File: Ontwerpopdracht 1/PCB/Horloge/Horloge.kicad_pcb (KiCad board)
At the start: 2 copper layers, 40 x 40 mm, 49 parts, among them J1 Conn_01x03, Q1 BSS138, U1 TPS613222ADBVT, U2 ATTINY414-SSF, Y1 FX135A-327

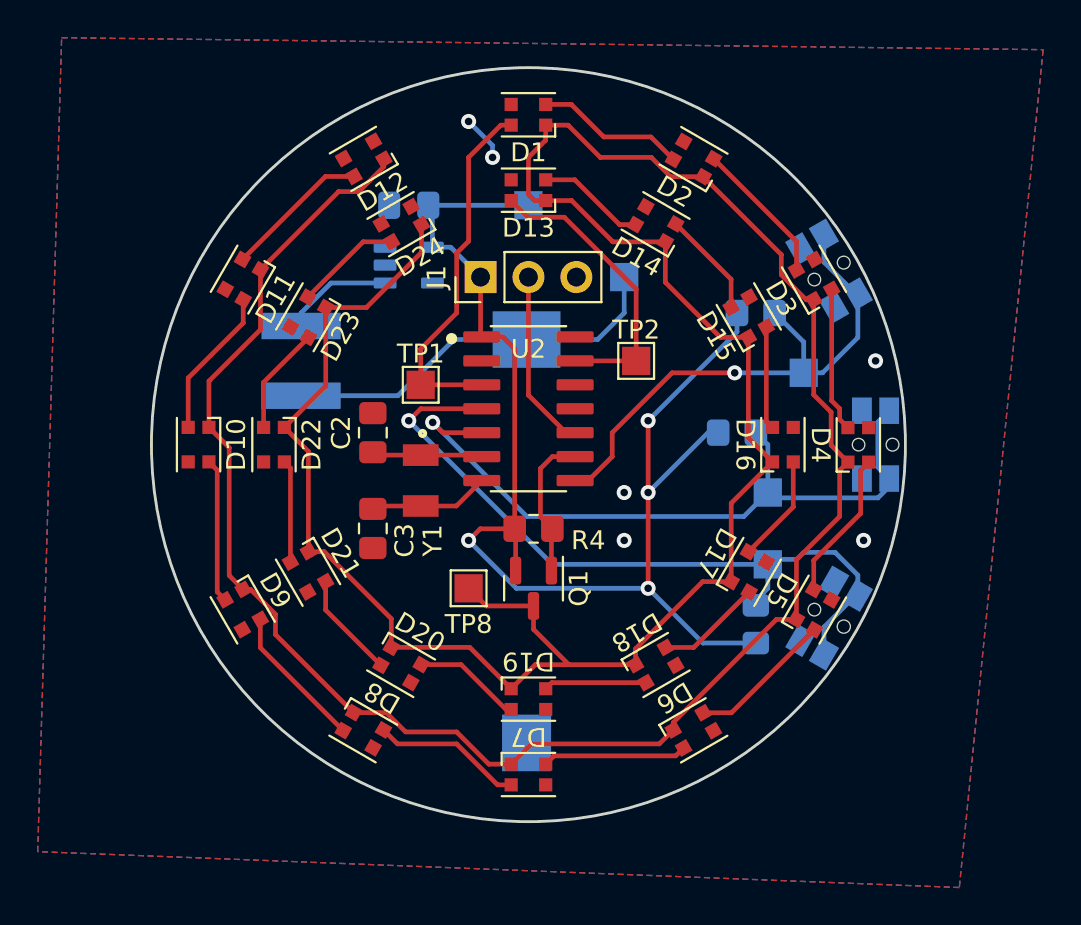
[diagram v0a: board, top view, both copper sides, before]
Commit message: pcb macropad klaar
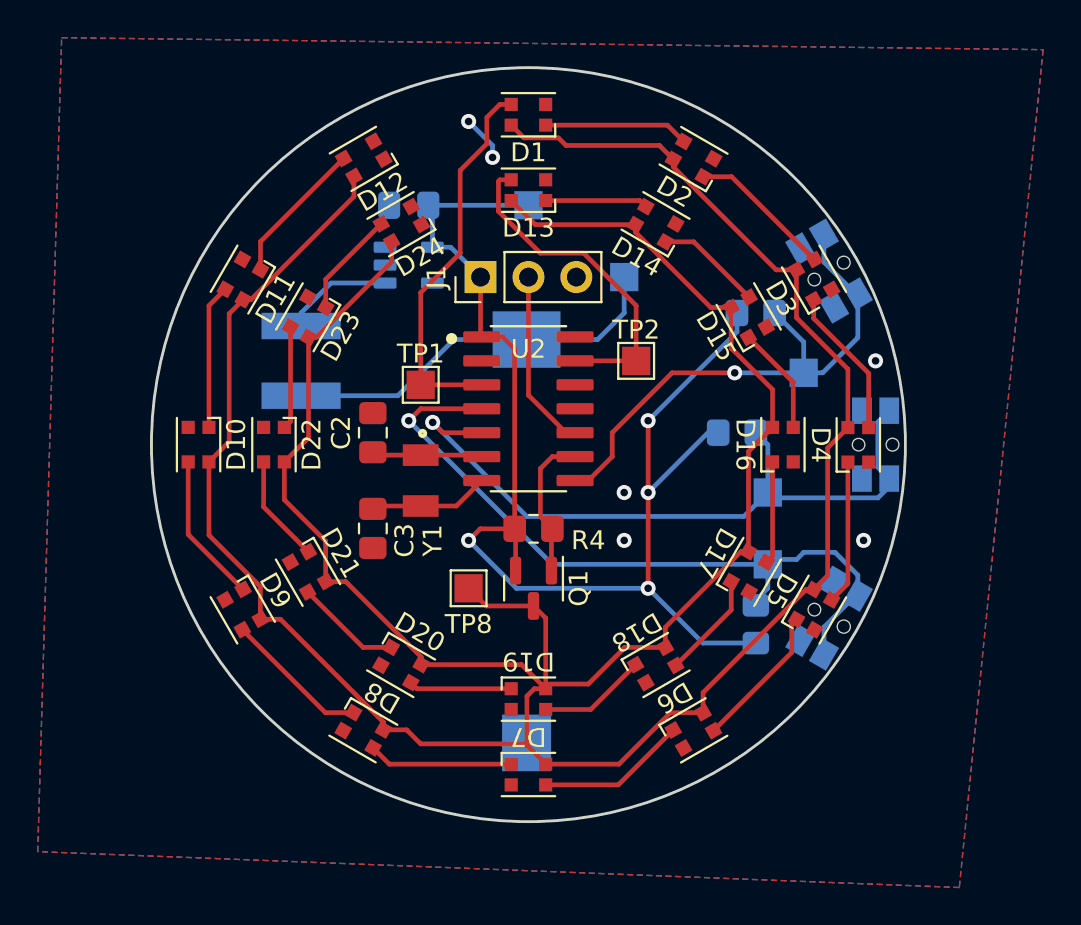
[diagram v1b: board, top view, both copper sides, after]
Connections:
- D1 pad 1: VDD -> Net-(D1-DOUT)
- D1 pad 2: Net-(D1-Pad2) -> GND
- D1 pad 3: GND -> LEDS UREN
- D1 pad 4: LEDS UREN -> VDD
- D10 pad 1: VDD -> Net-(D10-DOUT)
- D10 pad 2: Net-(D10-Pad2) -> GND
- D10 pad 3: GND -> Net-(D10-DIN)
- D10 pad 4: Net-(D10-Pad4) -> VDD
- D11 pad 1: VDD -> Net-(D11-DOUT)
- D11 pad 2: Net-(D11-Pad2) -> GND
- D11 pad 3: GND -> Net-(D10-DOUT)
- D11 pad 4: Net-(D10-Pad2) -> VDD
- D12 pad 1: VDD -> unconnected-(D12-DOUT-Pad1)
- D12 pad 2: unconnected-(D12-Pad2) -> GND
- D12 pad 3: GND -> Net-(D11-DOUT)
- D12 pad 4: Net-(D11-Pad2) -> VDD
- D13 pad 1: VDD -> Net-(D13-DOUT)
- D13 pad 2: Net-(D13-Pad2) -> GND
- D13 pad 3: GND -> LEDS MINUTEN
- D13 pad 4: LEDS MINUTEN -> VDD
- D14 pad 1: VDD -> Net-(D14-DOUT)
- D14 pad 2: Net-(D14-Pad2) -> GND
- D14 pad 3: GND -> Net-(D13-DOUT)
- D14 pad 4: Net-(D13-Pad2) -> VDD
- D15 pad 1: VDD -> Net-(D15-DOUT)
- D15 pad 2: Net-(D15-Pad2) -> GND
- D15 pad 3: GND -> Net-(D14-DOUT)
- D15 pad 4: Net-(D14-Pad2) -> VDD
- D16 pad 1: VDD -> Net-(D16-DOUT)
- D16 pad 2: Net-(D16-Pad2) -> GND
- D16 pad 3: GND -> Net-(D15-DOUT)
- D16 pad 4: Net-(D15-Pad2) -> VDD
- D17 pad 1: VDD -> Net-(D17-DOUT)
- D17 pad 2: Net-(D17-Pad2) -> GND
- D17 pad 3: GND -> Net-(D16-DOUT)
- D17 pad 4: Net-(D16-Pad2) -> VDD
- D18 pad 1: VDD -> Net-(D18-DOUT)
- D18 pad 2: Net-(D18-Pad2) -> GND
- D18 pad 3: GND -> Net-(D17-DOUT)
- D18 pad 4: Net-(D17-Pad2) -> VDD
- D19 pad 1: VDD -> Net-(D19-DOUT)
- D19 pad 2: Net-(D19-Pad2) -> GND
- D19 pad 3: GND -> Net-(D18-DOUT)
- D19 pad 4: Net-(D18-Pad2) -> VDD
- D2 pad 1: VDD -> Net-(D2-DOUT)
- D2 pad 2: Net-(D2-Pad2) -> GND
- D2 pad 3: GND -> Net-(D1-DOUT)
- D2 pad 4: Net-(D1-Pad2) -> VDD
- D20 pad 1: VDD -> Net-(D20-DOUT)
- D20 pad 2: Net-(D20-Pad2) -> GND
- D20 pad 3: GND -> Net-(D19-DOUT)
- D20 pad 4: Net-(D19-Pad2) -> VDD
- D21 pad 1: VDD -> Net-(D21-DOUT)
- D21 pad 2: Net-(D21-Pad2) -> GND
- D21 pad 3: GND -> Net-(D20-DOUT)
- D21 pad 4: Net-(D20-Pad2) -> VDD
- D22 pad 1: VDD -> Net-(D22-DOUT)
- D22 pad 2: Net-(D22-Pad2) -> GND
- D22 pad 3: GND -> Net-(D21-DOUT)
- D22 pad 4: Net-(D21-Pad2) -> VDD
- D23 pad 1: VDD -> Net-(D23-DOUT)
- D23 pad 2: Net-(D23-Pad2) -> GND
- D23 pad 3: GND -> Net-(D22-DOUT)
- D23 pad 4: Net-(D22-Pad2) -> VDD
- D24 pad 1: VDD -> unconnected-(D24-DOUT-Pad1)
- D24 pad 2: unconnected-(D24-Pad2) -> GND
- D24 pad 3: GND -> Net-(D23-DOUT)
- D24 pad 4: Net-(D23-Pad2) -> VDD
- D3 pad 1: VDD -> Net-(D3-DOUT)
- D3 pad 2: Net-(D3-Pad2) -> GND
- D3 pad 3: GND -> Net-(D2-DOUT)
- D3 pad 4: Net-(D2-Pad2) -> VDD
- D4 pad 1: VDD -> Net-(D4-DOUT)
- D4 pad 2: Net-(D4-Pad2) -> GND
- D4 pad 3: GND -> Net-(D3-DOUT)
- D4 pad 4: Net-(D3-Pad2) -> VDD
- D5 pad 1: VDD -> Net-(D5-DOUT)
- D5 pad 2: Net-(D5-Pad2) -> GND
- D5 pad 3: GND -> Net-(D4-DOUT)
- D5 pad 4: Net-(D4-Pad2) -> VDD
- D6 pad 1: VDD -> Net-(D6-DOUT)
- D6 pad 2: Net-(D6-Pad2) -> GND
- D6 pad 3: GND -> Net-(D5-DOUT)
- D6 pad 4: Net-(D5-Pad2) -> VDD
- D7 pad 1: VDD -> Net-(D7-DOUT)
- D7 pad 2: Net-(D7-Pad2) -> GND
- D7 pad 3: GND -> Net-(D6-DOUT)
- D7 pad 4: Net-(D6-Pad2) -> VDD
- D8 pad 1: VDD -> Net-(D8-DOUT)
- D8 pad 2: Net-(D8-Pad2) -> GND
- D8 pad 3: GND -> Net-(D7-DOUT)
- D8 pad 4: Net-(D7-Pad2) -> VDD
- D9 pad 1: VDD -> Net-(D10-DIN)
- D9 pad 2: Net-(D10-Pad4) -> GND
- D9 pad 3: GND -> Net-(D8-DOUT)
- D9 pad 4: Net-(D8-Pad2) -> VDD
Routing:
- net Net-(D3-DOUT): track 0.00 -> 7.99 mm
- net Net-(D1-Pad2): track 7.99 -> 0.00 mm
- net Net-(D7-Pad2): track 7.99 -> 0.00 mm
- net Net-(D10-Pad2): track 7.99 -> 0.00 mm
- net Net-(D6-DOUT): track 0.00 -> 7.97 mm
- net Net-(D10-DIN): track 0.00 -> 7.97 mm
- net Net-(D4-Pad2): track 7.97 -> 0.00 mm
- net Net-(D11-Pad2): track 7.74 -> 0.00 mm
- net Net-(D11-DOUT): track 0.00 -> 7.73 mm
- net Net-(D5-Pad2): track 7.73 -> 0.00 mm
- net Net-(D5-DOUT): track 0.00 -> 7.73 mm
- net Net-(D8-Pad2): track 7.73 -> 0.00 mm
- net Net-(D8-DOUT): track 0.00 -> 7.72 mm
- net Net-(D2-Pad2): track 7.72 -> 0.00 mm
- net Net-(D2-DOUT): track 0.00 -> 7.72 mm
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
